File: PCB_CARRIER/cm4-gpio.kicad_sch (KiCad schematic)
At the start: 18 parts, among them J2 Micro_SD_Card_Det2, Q1 BSS138, SW4 SW_DIP_x04, U1 RT9742GGJ5

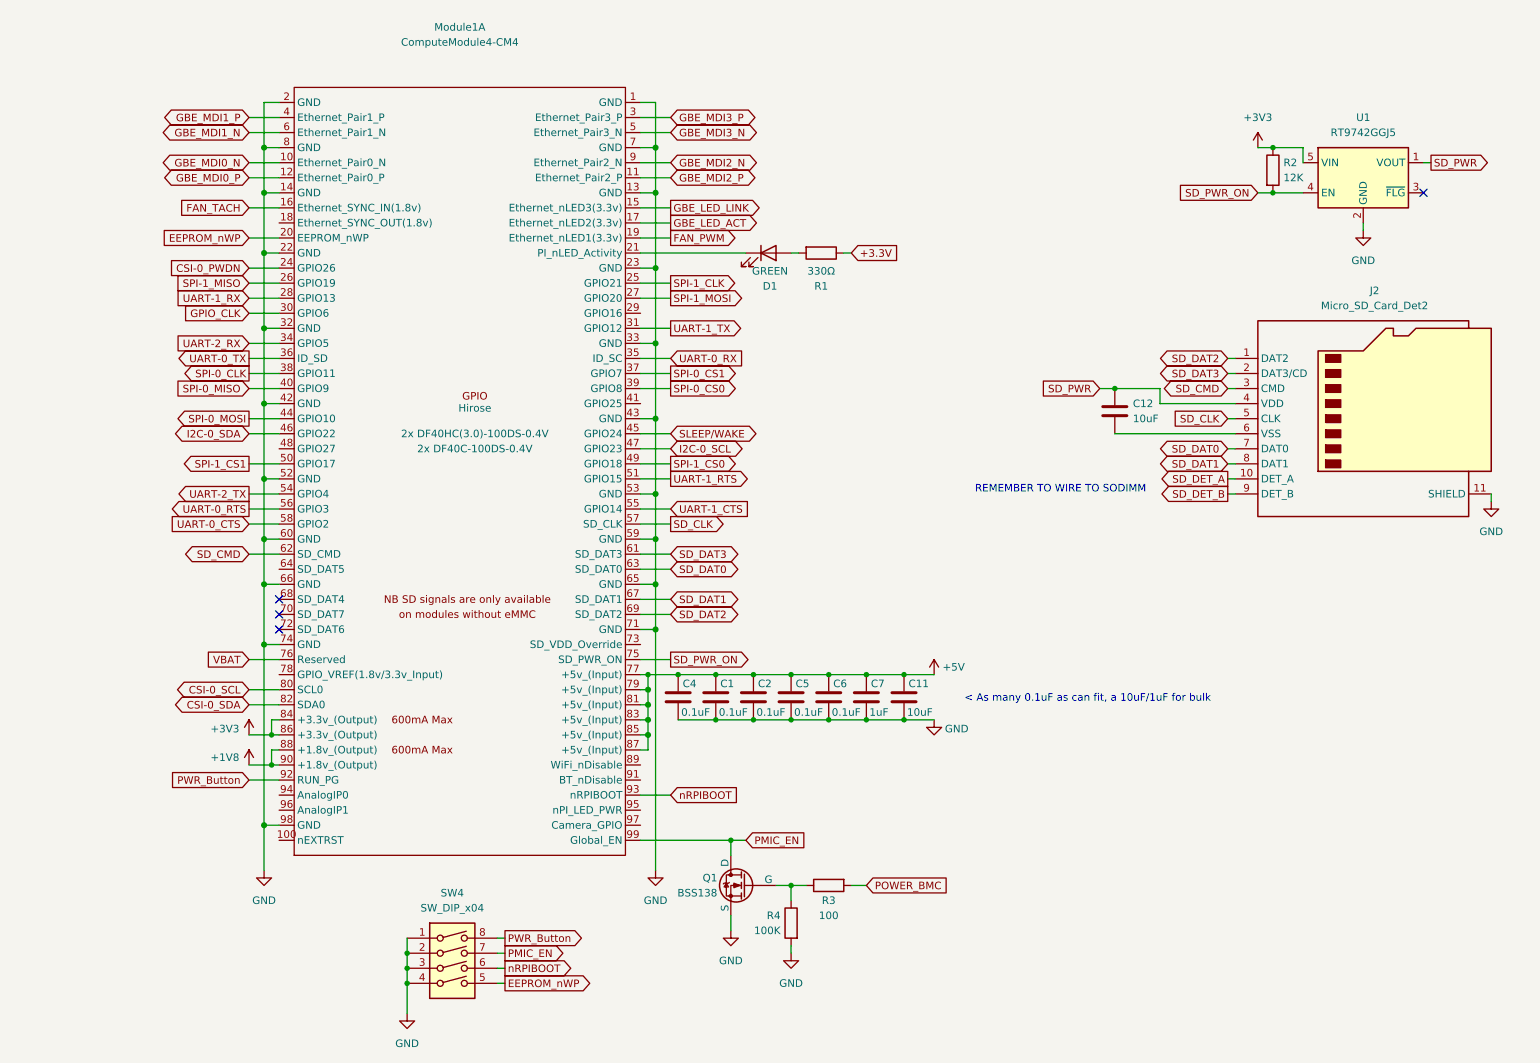
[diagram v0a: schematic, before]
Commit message: added system reset
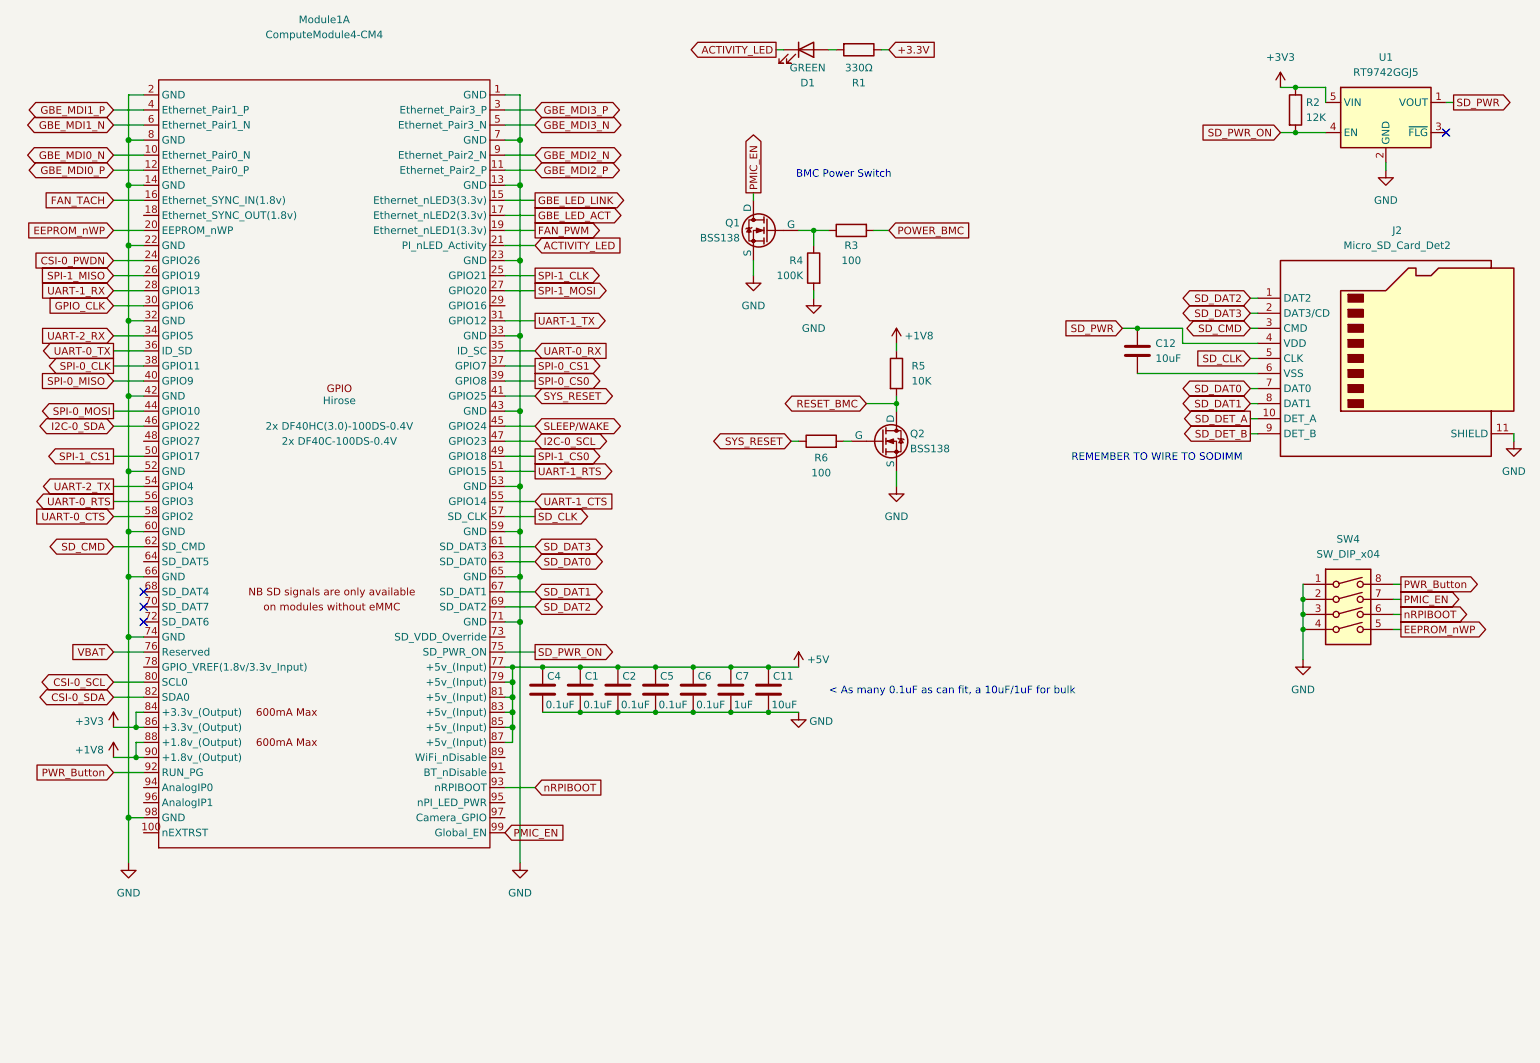
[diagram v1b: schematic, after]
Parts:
- added Q2: BSS138, symbol Simulation_SPICE:NMOS
- added R5: 10K, symbol Device:R
- added R6: 100, symbol Device:R
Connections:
- net +1V8: now also R5.1
- net GND: now also Q2.3 (S)
- net ACTIVITY_LED: now reaches D1.1 (K), Module1.21 (PI_nLED_Activity)
- net SYS_RESET: now reaches Module1.41 (GPIO25)
- net SYS_RESET: now also R6.1
- new net: Q2.2 (G), R6.2
- new net RESET_BMC: Q2.1 (D), R5.2
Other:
- note added: "BMC Power Switch"
- moved on the sheet: C1, C11, C12, C2, C4, C5, C6, C7, D1, J2, Module1A, Q1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
